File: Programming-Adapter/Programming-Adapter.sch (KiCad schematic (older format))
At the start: 1 part, among them J3 6P6C

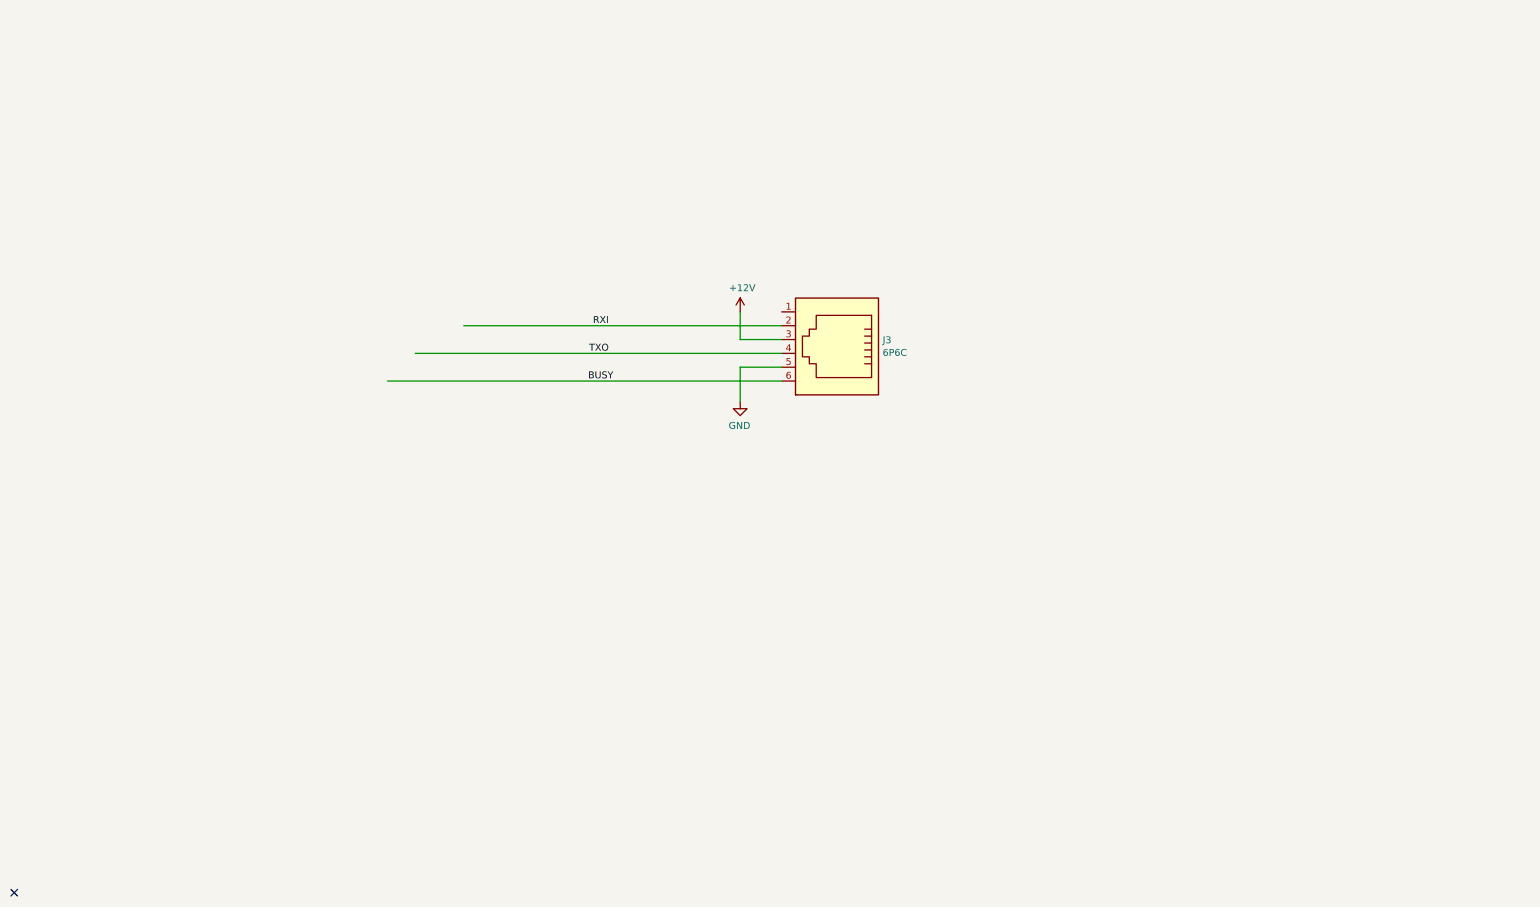
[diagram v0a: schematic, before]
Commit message: adapter
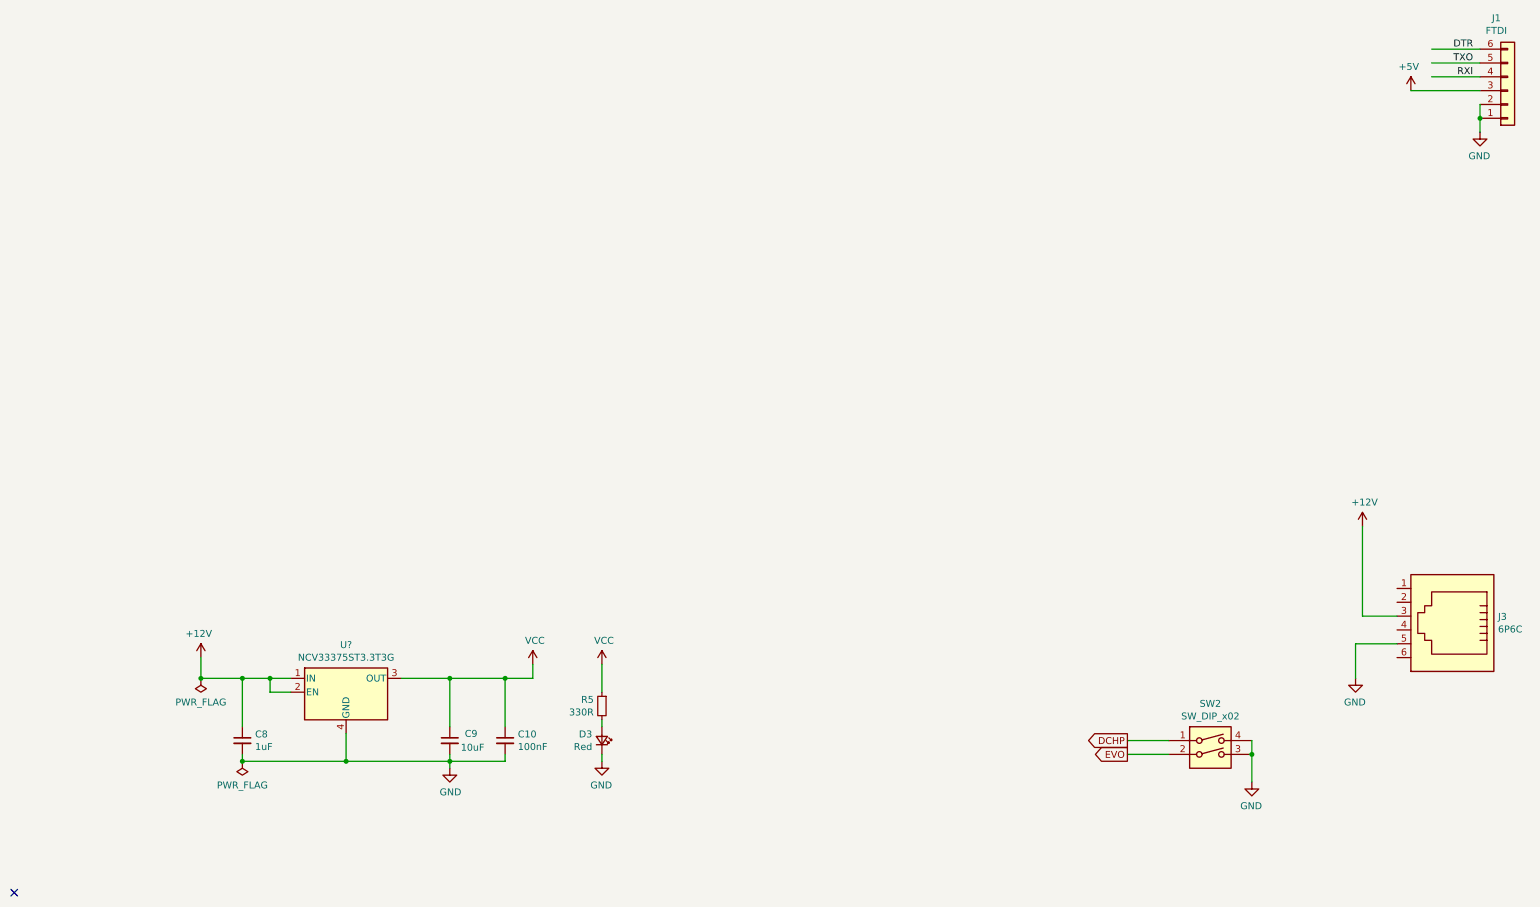
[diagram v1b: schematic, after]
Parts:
- added C10: 100nF, Capacitor_SMD:C_0603_1608Metric, symbol Device:C_Small
- added C8: 1uF, Capacitor_SMD:C_0603_1608Metric, symbol Device:C_Small
- added C9: 10uF, Capacitor_SMD:C_0603_1608Metric, symbol Device:C_Small
- added D3: Red, LED_SMD:LED_0603_1608Metric, symbol Device:LED_Small
- added J1: FTDI, Connector_PinHeader_2.54mm:PinHeader_1x06_P2.54mm_Horizontal, symbol Connector_Generic:Conn_01x06
- added R5: 330R, Resistor_SMD:R_0603_1608Metric, symbol Device:R_Small
- added SW2: SW_DIP_x02, Button_Switch_SMD:SW_DIP_SPSTx02_Slide_6.7x6.64mm_W8.61mm_P2.54mm_LowProfile, symbol Switch:SW_DIP_x02
- added U?: NCV33375ST3.3T3G, Package_TO_SOT_SMD:SOT-223, symbol Regulator_Linear:NCV33375ST3.3T3G
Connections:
- net labels added: +5V, DCHP, DTR, EVO, VCC
- net labels removed: BUSY
- wire segments 7 -> 38

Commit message: programming adapter
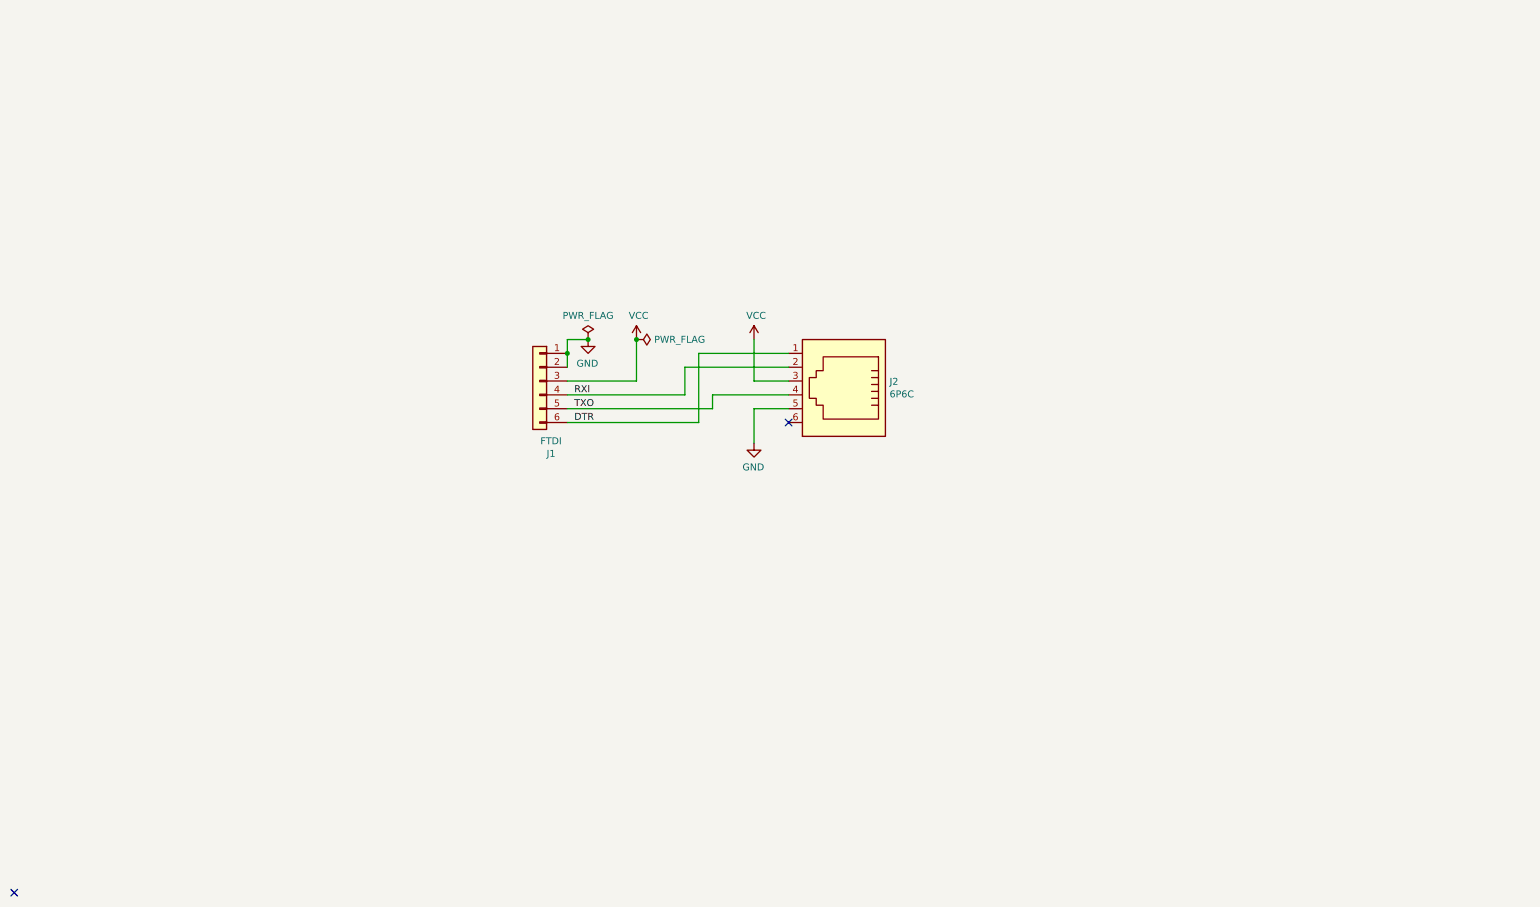
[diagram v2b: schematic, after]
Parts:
- removed C10: 100nF, Capacitor_SMD:C_0603_1608Metric, symbol Device:C_Small
- removed C8: 1uF, Capacitor_SMD:C_0603_1608Metric, symbol Device:C_Small
- removed C9: 10uF, Capacitor_SMD:C_0603_1608Metric, symbol Device:C_Small
- removed D3: Red, LED_SMD:LED_0603_1608Metric, symbol Device:LED_Small
- removed R5: 330R, Resistor_SMD:R_0603_1608Metric, symbol Device:R_Small
- removed SW2: SW_DIP_x02, Button_Switch_SMD:SW_DIP_SPSTx02_Slide_6.7x6.64mm_W8.61mm_P2.54mm_LowProfile, symbol Switch:SW_DIP_x02
- removed U?: NCV33375ST3.3T3G, Package_TO_SOT_SMD:SOT-223, symbol Regulator_Linear:NCV33375ST3.3T3G
- renumbered J3 to J2
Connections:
- net labels removed: +12V, +5V, DCHP, EVO
- wire segments 38 -> 18
- no-connect marks 1 -> 2
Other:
- moved on the sheet: J1, J2

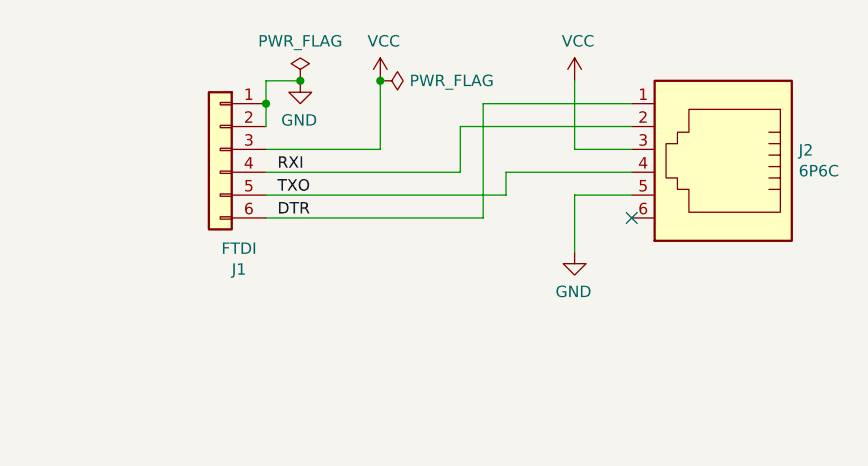
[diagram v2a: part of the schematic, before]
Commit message: update
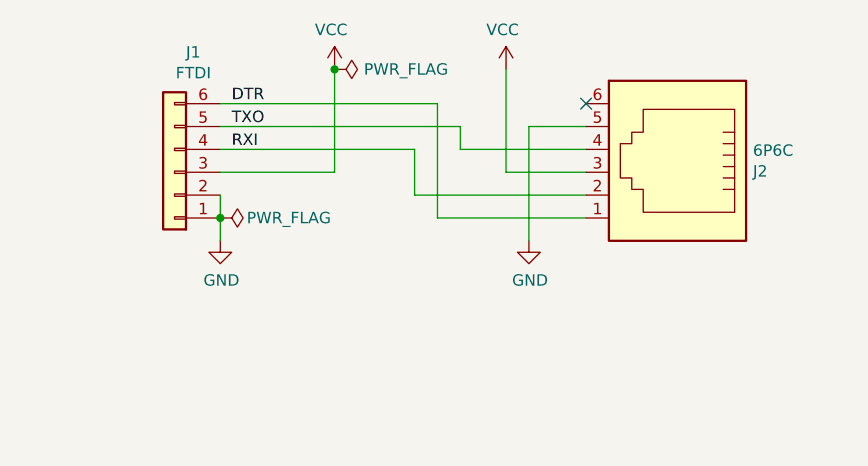
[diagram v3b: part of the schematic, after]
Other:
- moved on the sheet: J1, J2
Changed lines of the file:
@@
 L Connector:6P6C J2
 U 1 1 619B111F
-P 6250 3200
-F 0 "J2" H 5920 3204 50  0000 R CNN
-F 1 "6P6C" H 5920 3295 50  0000 R CNN
-F 2 "Connector_RJ:RJ12_Amphenol_54601" V 6250 3225 50  0001 C CNN
-F 3 "~" V 6250 3225 50  0001 C CNN
-F 4 "54601-906001WPLF" H 6250 3200 50  0001 C CNN "MPN"
-F 5 "Amphenol" H 6250 3200 50  0001 C CNN "Manufacturer"
-	1    6250 3200
-	-1   0    0    1
+P 6050 3300
+F 0 "J2" H 5720 3304 50  0000 R CNN
+F 1 "6P6C" H 5720 3395 50  0000 R CNN
+F 2 "Connector_RJ:RJ12_Amphenol_54601" V 6050 3325 50  0001 C CNN
+F 3 "~" V 6050 3325 50  0001 C CNN
+F 4 "54601-906001WPLF" H 6050 3300 50  0001 C CNN "MPN"
+F 5 "Amphenol" H 6050 3300 50  0001 C CNN "Manufacturer"
+	1    6050 3300
+	-1   0    0    -1
 $EndComp
 $Comp
 L power:GND #PWR04
 U 1 1 619B1120
-P 5600 3650
-F 0 "#PWR04" H 5600 3400 50  0001 C CNN
-F 1 "GND" H 5605 3477 50  0000 C CNN
-F 2 "" H 5600 3650 50  0001 C CNN
-F 3 "" H 5600 3650 50  0001 C CNN
-	1    5600 3650
-	-1   0    0    -1
+P 5400 3600
+F 0 "#PWR04" H 5400 3350 50  0001 C CNN
+F 1 "GND" H 5405 3427 50  0000 C CNN
+F 2 "" H 5400 3600 50  0001 C CNN
+F 3 "" H 5400 3600 50  0001 C CNN
+	1    5400 3600
+	1    0    0    -1
 $EndComp
 $Comp
 L Connector_Generic:Conn_01x06 J1
 U 1 1 61AF9A7D
-P 4050 3200
-F 0 "J1" H 3968 2675 50  0000 C CNN
-F 1 "FTDI" H 3968 2766 50  0000 C CNN
-F 2 "Connector_PinHeader_2.54mm:PinHeader_1x06_P2.54mm_Horizontal" H 4050 3200 50  0001 C CNN
-F 3 "~" H 4050 3200 50  0001 C CNN
-	1    4050 3200
+P 3850 3300
+F 0 "J1" H 3768 2775 50  0000 C CNN
+F 1 "FTDI" H 3768 2866 50  0000 C CNN
+F 2 "Connector_PinHeader_2.54mm:PinHeader_1x06_P2.54mm_Horizontal" H 3850 3300 50  0001 C CNN
+F 3 "~" H 3850 3300 50  0001 C CNN
+	1    3850 3300
+	-1   0    0    1
+$EndComp
+Text Label 4100 3000 0    50   ~ 0
+DTR
+Text Label 4100 3100 0    50   ~ 0
+TXO
+Text Label 4100 3200 0    50   ~ 0
+RXI
+$Comp
+L power:GND #PWR03
+U 1 1 61BBCFD8
+P 4050 3600
+F 0 "#PWR03" H 4050 3350 50  0001 C CNN
+F 1 "GND" H 4055 3427 50  0000 C CNN
+F 2 "" H 4050 3600 50  0001 C CNN
+F 3 "" H 4050 3600 50  0001 C CNN
+	1    4050 3600
+	1    0    0    -1
+$EndComp
+Wire Wire Line
+	5650 3100 5400 3100
+Wire Wire Line
+	4050 3400 4050 3500
+Connection ~ 4050 3500
+Wire Wire Line
+	4050 3600 4050 3500
+NoConn ~ 250  6900
+$Comp
+L power:VCC #PWR01
+U 1 1 619CC009
+P 4550 2850
+F 0 "#PWR01" H 4550 2700 50  0001 C CNN
+F 1 "VCC" H 4565 3023 50  0000 C CNN
+F 2 "" H 4550 2850 50  0001 C CNN
+F 3 "" H 4550 2850 50  0001 C CNN
+	1    4550 2850
 	-1   0    0    -1
 $EndComp
-Text Label 4300 3500 0    50   ~ 0
-DTR
-Text Label 4300 3400 0    50   ~ 0
-TXO
-Text Label 4300 3300 0    50   ~ 0
-RXI
 $Comp
-L power:GND #PWR01
-U 1 1 61BBCFD8
-P 4400 2900
-F 0 "#PWR01" H 4400 2650 50  0001 C CNN
-F 1 "GND" H 4405 2727 50  0000 C CNN
-F 2 "" H 4400 2900 50  0001 C CNN
-F 3 "" H 4400 2900 50  0001 C CNN
-	1    4400 2900
+L power:VCC #PWR02
+U 1 1 619CC80D
+P 5300 2850
+F 0 "#PWR02" H 5300 2700 50  0001 C CNN
+F 1 "VCC" H 5315 3023 50  0000 C CNN
+F 2 "" H 5300 2850 50  0001 C CNN
+F 3 "" H 5300 2850 50  0001 C CNN
+	1    5300 2850
 	-1   0    0    -1
 $EndComp
 Wire Wire Line
-	5850 3400 5600 3400
+	5650 3500 5000 3500
 Wire Wire Line
-	4250 3100 4250 3000
-Connection ~ 4250 3000
+	5000 3500 5000 3000
 Wire Wire Line
-	4250 2900 4250 3000
-NoConn ~ 250  6900
+	4050 3000 5000 3000
 Wire Wire Line
-	5850 3200 5600 3200
+	4900 3200 4900 3400
 Wire Wire Line
-	5600 2900 5600 3200
+	4900 3400 5650 3400
 Wire Wire Line
-	4250 2900 4400 2900
+	4050 3200 4900 3200
+Wire Wire Line
+	5100 3100 5100 3200
+Wire Wire Line
+	5100 3200 5650 3200
+Wire Wire Line
+	4050 3100 5100 3100
+NoConn ~ 5650 3000
 $Comp
-L power:VCC #PWR02
-U 1 1 619CC009
-P 4750 2900
-F 0 "#PWR02" H 4750 2750 50  0001 C CNN
-F 1 "VCC" H 4765 3073 50  0000 C CNN
-F 2 "" H 4750 2900 50  0001 C CNN
-F 3 "" H 4750 2900 50  0001 C CNN
-	1    4750 2900
-	1    0    0    -1
-$EndComp
-$Comp
-L power:VCC #PWR03
-U 1 1 619CC80D
-P 5600 2900
-F 0 "#PWR03" H 5600 2750 50  0001 C CNN
-F 1 "VCC" H 5615 3073 50  0000 C CNN
-F 2 "" H 5600 2900 50  0001 C CNN
-F 3 "" H 5600 2900 50  0001 C CNN
-	1    5600 2900
-	1    0    0    -1
+L power:PWR_FLAG #FLG02
+U 1 1 619CF64E
+P 4050 3500
+F 0 "#FLG02" H 4050 3575 50  0001 C CNN
+F 1 "PWR_FLAG" V 4050 3800 50  0000 C CNN
+F 2 "" H 4050 3500 50  0001 C CNN
+F 3 "~" H 4050 3500 50  0001 C CNN
+	1    4050 3500
+	0    1    -1   0
 $EndComp
 Wire Wire Line
-	5850 3000 5200 3000
-Wire Wire Line
-	5200 3000 5200 3500
-Wire Wire Line
-	4250 3500 5200 3500
-Wire Wire Line
-	5100 3300 5100 3100
-Wire Wire Line
-	5100 3100 5850 3100
-Wire Wire Line
-	4250 3300 5100 3300
-Wire Wire Line
-	5300 3400 5300 3300
-Wire Wire Line
-	5300 3300 5850 3300
-Wire Wire Line
-	4250 3400 5300 3400
-NoConn ~ 5850 3500
-Wire Wire Line
-	5600 3650 5600 3400
+	4050 3300 4550 3300
 $Comp
 L power:PWR_FLAG #FLG01
-U 1 1 619CF64E
-P 4400 2900
-F 0 "#FLG01" H 4400 2975 50  0001 C CNN
-F 1 "PWR_FLAG" H 4400 3073 50  0000 C CNN
-F 2 "" H 4400 2900 50  0001 C CNN
-F 3 "~" H 4400 2900 50  0001 C CNN
-	1    4400 2900
-	1    0    0    -1
+U 1 1 619D0642
+P 4550 2850
+F 0 "#FLG01" H 4550 2925 50  0001 C CNN
+F 1 "PWR_FLAG" V 4550 2978 50  0000 L CNN
+F 2 "" H 4550 2850 50  0001 C CNN
+F 3 "~" H 4550 2850 50  0001 C CNN
+	1    4550 2850
+	0    1    -1   0
 $EndComp
-Connection ~ 4400 2900
 Wire Wire Line
-	4750 3200 4750 2900
+	4550 3300 4550 2850
+Connection ~ 4550 2850
 Wire Wire Line
-	4250 3200 4750 3200
-$Comp
-L power:PWR_FLAG #FLG02
-U 1 1 619D0642
-P 4750 2900
-F 0 "#FLG02" H 4750 2975 50  0001 C CNN
-F 1 "PWR_FLAG" V 4750 3028 50  0000 L CNN
-F 2 "" H 4750 2900 50  0001 C CNN
-F 3 "~" H 4750 2900 50  0001 C CNN
-	1    4750 2900
-	0    1    1    0
-$EndComp
-Connection ~ 4750 2900
+	5300 3300 5300 2850
+Wire Wire Line
+	5300 3300 5650 3300
+Wire Wire Line
+	5400 3100 5400 3600
 $EndSCHEMATC
